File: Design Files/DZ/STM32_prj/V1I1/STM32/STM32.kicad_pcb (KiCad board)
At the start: 4 copper layers, 60 x 16.5 mm, 41 parts, among them J1 Conn_01x04, J2 Conn_Coaxial, J3 USB_C_Receptacle_USB2.0_16P, J4 Conn_ARM_SWD_TagConnect_TC2030, SW1 SW_Push, U1 MIC5365-3.3YD5, U2 USBLC6-2SC6, U3 STM32WB55CEUx, X1 32MHz, X2 32kHz768

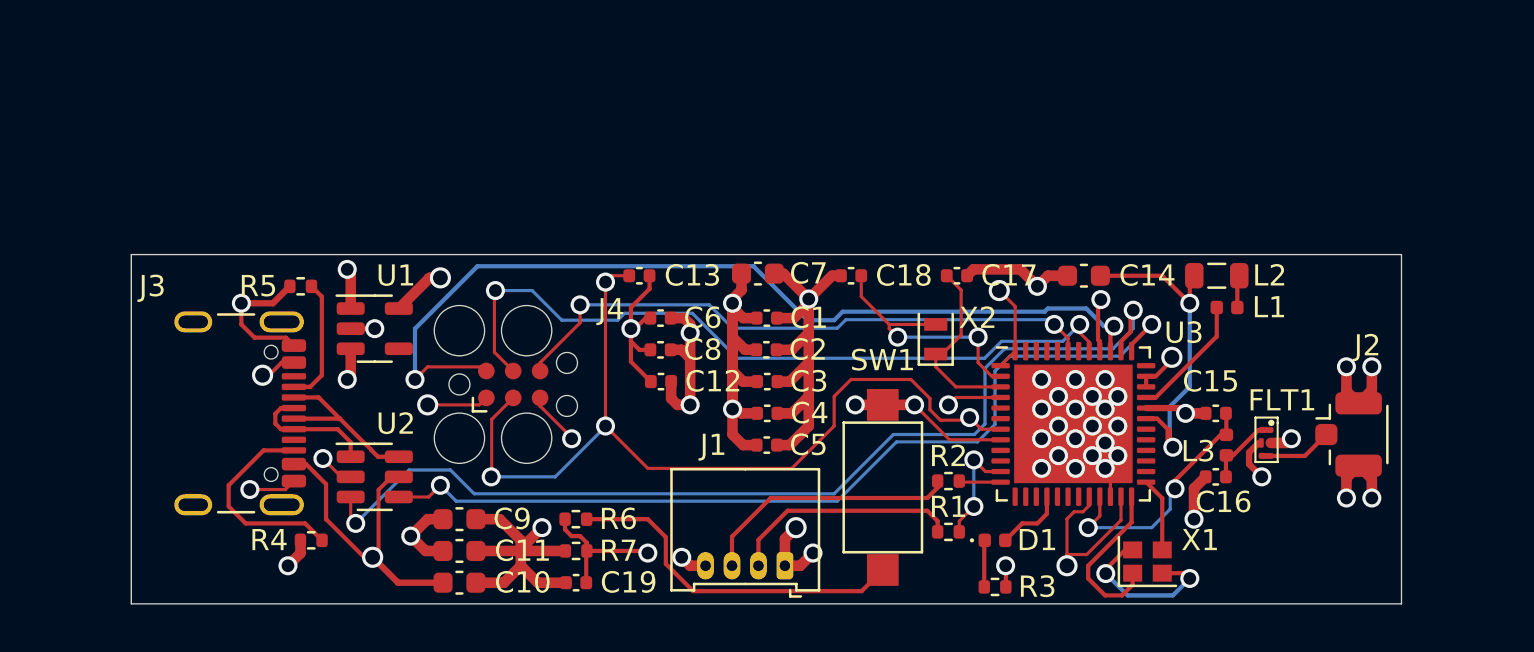
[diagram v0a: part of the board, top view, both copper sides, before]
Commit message: Update 03
Project accomplished
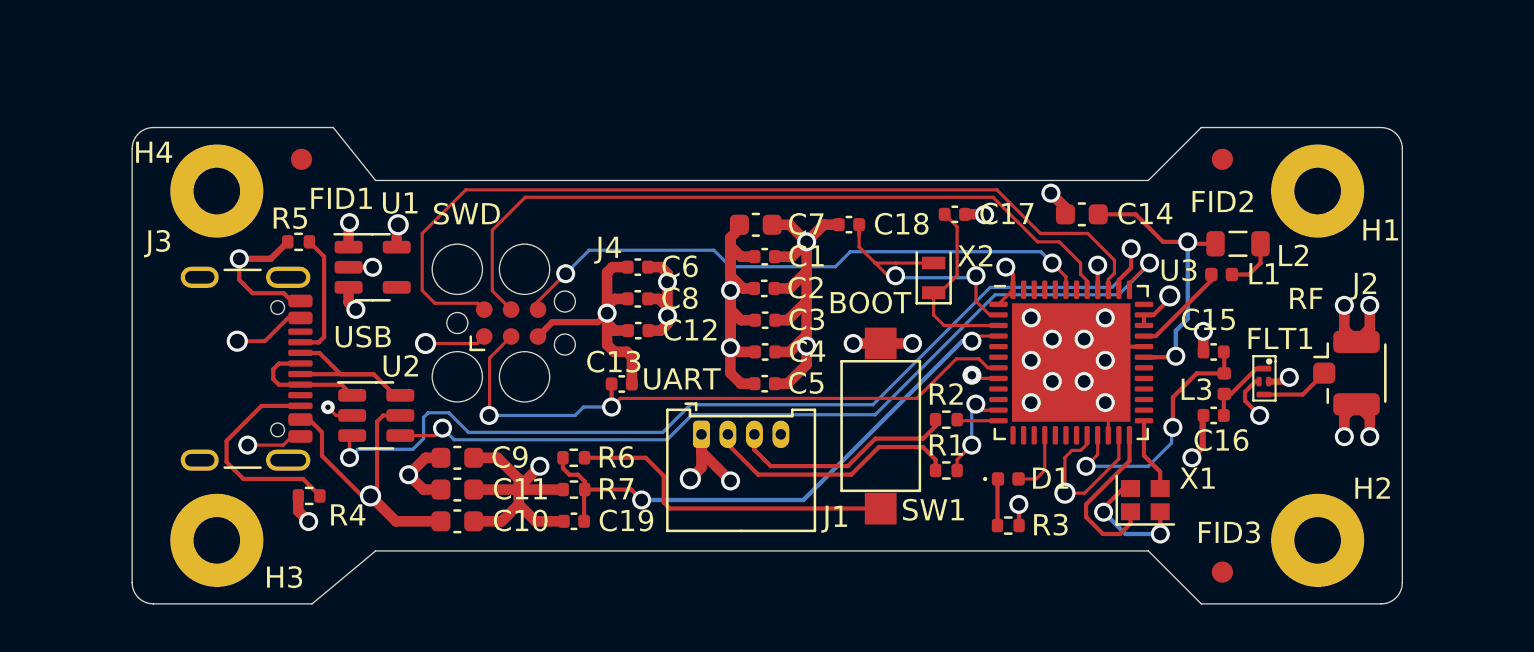
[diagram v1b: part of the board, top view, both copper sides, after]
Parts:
- added FID1: Fiducial, Fiducial:Fiducial_1mm_Mask2mm, F.Cu at (126.5, 49.0)
- added FID2: Fiducial, Fiducial:Fiducial_1mm_Mask2mm, F.Cu at (170.0, 49.0)
- added FID3: Fiducial, Fiducial:Fiducial_1mm_Mask2mm, F.Cu at (170.0, 68.5)
- added H1: MountingHole_Pad, MountingHole:MountingHole_2.2mm_M2_Pad, F.Cu at (174.5, 50.5)
- added H2: MountingHole_Pad, MountingHole:MountingHole_2.2mm_M2_Pad, F.Cu at (174.5, 67.0)
- added H3: MountingHole_Pad, MountingHole:MountingHole_2.2mm_M2_Pad, F.Cu at (122.5, 67.0)
- added H4: MountingHole_Pad, MountingHole:MountingHole_2.2mm_M2_Pad, F.Cu at (122.5, 50.5)
- moved J1 7.35 mm to (145.4, 62.0), turned to 0 degrees
- moved C13 5.18 mm to (141.6, 59.6)
- moved D1 2.97 mm to (159.9, 64.1)
- moved R3 2.97 mm to (159.9, 66.3)
- moved C10 2.90 mm to (133.9, 66.1)
- moved C11 2.90 mm to (133.9, 64.6)
- moved C19 2.90 mm to (139.4, 66.1)
- moved R2 2.90 mm to (157.0, 61.3)
- moved R7 2.90 mm to (139.4, 64.6)
- moved X1 2.90 mm to (166.4, 65.1)
- moved C1 2.90 mm to (148.4, 53.6)
- moved C14 2.90 mm to (163.4, 51.6)
- moved C15 2.90 mm to (169.6, 58.1)
- moved C16 2.90 mm to (169.6, 61.1)
- moved C17 2.90 mm to (157.4, 51.6)
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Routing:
- net /BOOT: track 9.20 -> 26.6 mm
- net /SWD_NRST: track 42.1 -> 30.6 mm, vias 4 -> 2
- net +3V3: track 68.9 -> 58.6 mm, vias 15 -> 16
- net Net-(X1-Pad2): track 7.98 -> 6.01 mm
- net /SMPS_FB: track 15.6 -> 13.8 mm
- net /USB_D-: track 42.7 -> 40.9 mm
- net /UART_RXC: track 12.4 -> 10.7 mm
- net /USBC_D-: track 8.30 -> 9.83 mm
- net /SMPSLX: track 5.90 -> 4.55 mm
- net /UART_TXC: track 11.0 -> 12.2 mm
- net /USB_D+: track 47.4 -> 46.4 mm
- net /SMPSLXL: track 1.54 -> 2.48 mm
- net Net-(R6-Pad1): track 16.6 -> 15.7 mm
- net GND: track 82.1 -> 82.9 mm, vias 41 -> 30
- net /RF: track 11.7 -> 12.3 mm
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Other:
- board size 60 x 16.5 mm -> 60 x 22.5 mm
- rule pad_to_mask_clearance: 0.8 -> 0
- board text added: "02-24-2024"
- board text added: "BOOT"
- board text added: "DJAMAL ZILAL"
- board text added: "RF"
- board text added: "STM32WB - Rev01"
- board text added: "SWD"
- board text added: "UART"
- board text added: "USB"
